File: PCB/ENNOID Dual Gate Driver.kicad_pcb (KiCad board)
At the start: 2 copper layers, 60 x 98 mm, 138 parts, among them J1 Conn_02x08_Odd_Even, J2 Current, J3 TEMP, J4 PHASE, J5 Collector, J6 Gate_H, J7 G_L, J8 E, M1 MountingHole_2.2mm_M2_Pad_Via, M2 MountingHole_2.2mm_M2_Pad_Via, M3 MountingHole_2.2mm_M2_Pad_Via, Q1 Q_NPN_BCE, Q2 Q_NPN_BCE, Q3 2N7002K-7, Q4 2N7002K-7, Q5 2N7002, Q6 2N7002, Q7 2N7002, Q8 2N7002, U1 MC7805, U2 MGJ2, U3 MGJ2, U4 1ED020I12-F2, U5 IXD-609, U6 1ED020I12-F2, U7 IXD-609, U8 AMC1301, U9 4069

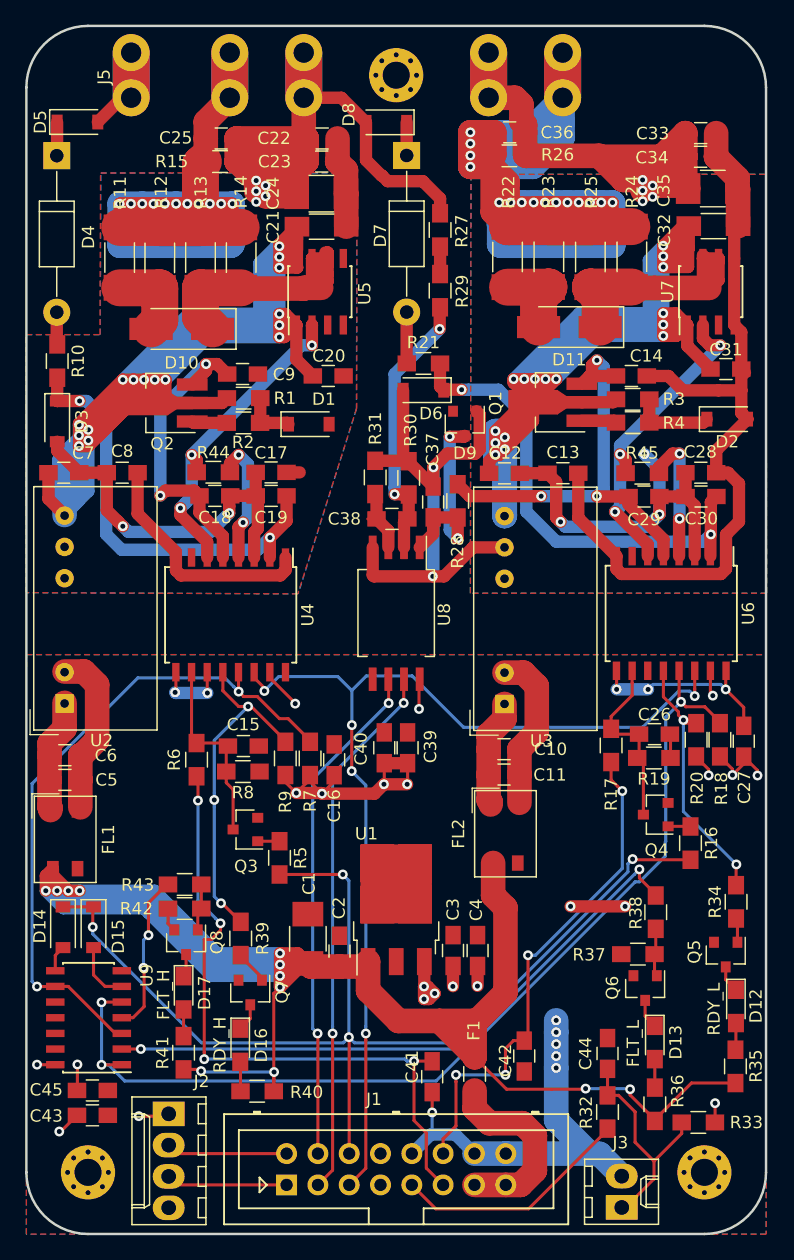
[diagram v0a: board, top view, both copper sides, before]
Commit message: PCB changes
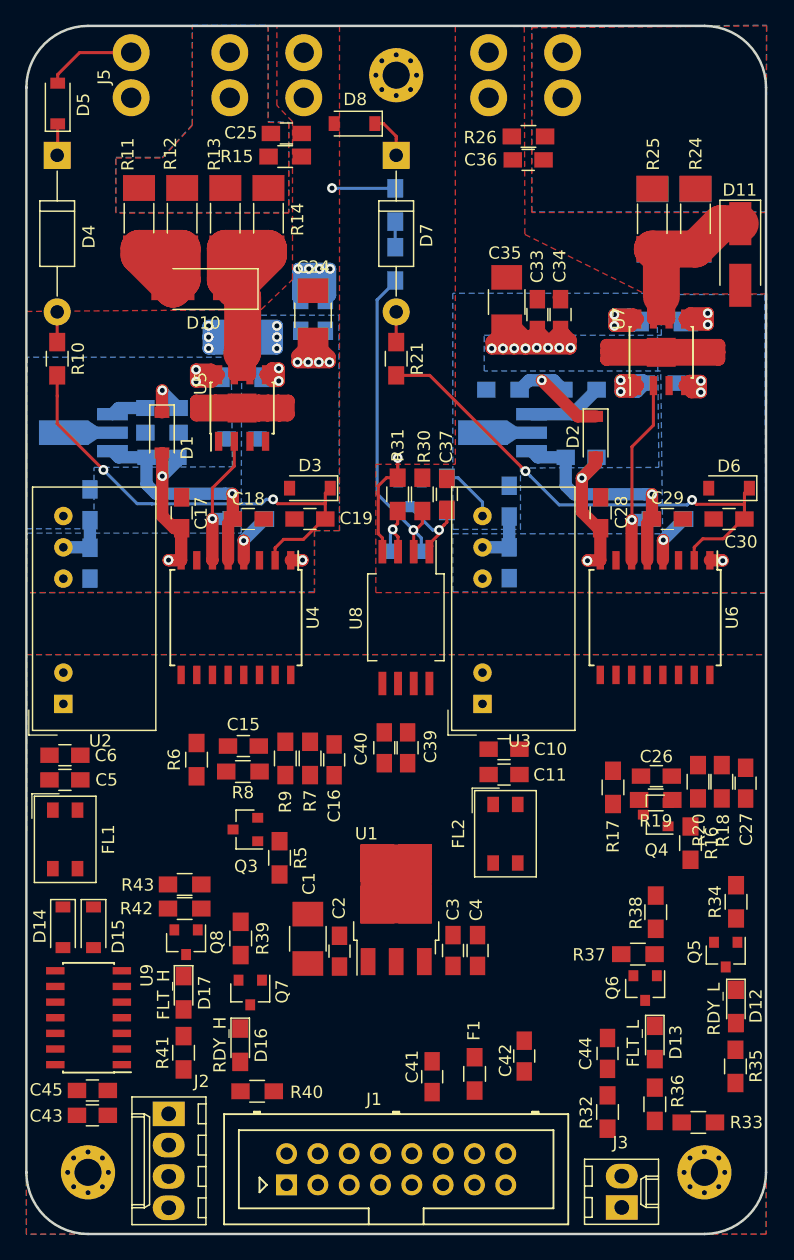
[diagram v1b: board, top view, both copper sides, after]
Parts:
- C12, C13, C14, C20, C21, C22, C23, C31, C32, C38, C7, C8, C9, D9, Q1, Q2, R1, R2, R22, R23, R27, R28, R29, R3, R4, R44, R45: moved to B.Cu
- R19, R8: value 1k -> 47k
- U5, U7: footprint Housings_SOIC:SOIC-8_3.9x4.9mm_Pitch1.27mm -> Housings_SOIC:SOIC-8-1EP_3.9x4.9mm_Pitch1.27mm
- moved D6 26.0 mm to (57.0, 37.5)
- moved D3 21.2 mm to (23.0, 37.5), turned to 180 degrees
- moved C33 19.8 mm to (41.5, 23.4), turned to 270 degrees
- moved C35 19.1 mm to (39.0, 22.4), turned to 270 degrees
- moved C34 17.1 mm to (43.3, 23.4), turned to 270 degrees
- moved D11 15.1 mm to (57.9, 18.5), turned to 270 degrees
- moved C22 14.4 mm to (24.3, 23.5), turned to 270 degrees
- moved C21 13.8 mm to (17.5, 28.5)
- moved C23 12.6 mm to (22.3, 23.5), turned to 270 degrees
- moved R23 12.3 mm to (54.3, 15.7)
- moved R22 12.1 mm to (50.8, 15.7)
- moved D1 11.9 mm to (11.0, 33.0), turned to 270 degrees
- moved U5 11.3 mm to (17.5, 31.0)
- moved D2 10.8 mm to (46.2, 33.3), turned to 270 degrees
- moved R3 10.6 mm to (38.7, 29.5)
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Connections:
- R28 pad 2: /GD_LOW/VCC_REG -> /GD_LOW/+VCC
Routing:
- net /GD_HIGH/+VCC: track 209.5 -> 5.02 mm, vias 16 -> 2
- net VCC_IN: track 182.9 -> 0.00 mm, vias 12 -> 0
- net /GD_LOW/+VCC: track 181.8 -> 25.1 mm, vias 16 -> 4
- net /GD_LOW/G: track 144.7 -> 0.00 mm, vias 15 -> 0
- net /GD_LOW/E: track 123.8 -> 15.8 mm, vias 10 -> 1
- net /GD_HIGH/G: track 93.5 -> 0.00 mm, vias 11 -> 0
- net FLT_ALL: track 91.8 -> 0.00 mm, vias 4 -> 0
- net RST: track 84.5 -> 0.00 mm, vias 5 -> 0
- net FLT_L: track 81.8 -> 0.00 mm, vias 3 -> 0
- net GND: track 62.1 -> 0.00 mm, vias 11 -> 0
- net +5V: track 61.7 -> 0.00 mm, vias 22 -> 0
- net FLT_H: track 55.9 -> 0.00 mm, vias 2 -> 0
- net PWM_H: track 54.2 -> 0.00 mm, vias 4 -> 0
- net (no net): track 0.00 -> 53.0 mm
- net Net-(R38-Pad1): track 50.7 -> 0.00 mm, vias 2 -> 0
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- added copper zone on B.Cu, net /GD_HIGH/+VCC
- added copper zone on B.Cu, net /GD_HIGH/-VEE
- added copper zone on B.Cu, net /GD_HIGH/G
- added copper zone on F.Cu, net /GD_HIGH/G
- added copper zone on B.Cu, net /GD_LOW/+VCC
- added copper zone on B.Cu, net /GD_LOW/-VEE
- added copper zone on F.Cu, net /GD_LOW/E
- added copper zone on B.Cu, net /GD_LOW/G
- added copper zone on F.Cu, net /GD_LOW/G
- added copper zone on F.Cu, net PHASE
- removed copper zone on F.Cu, net /GD_HIGH/-VEE
- removed copper zone on F.Cu, net /GD_LOW/-VEE
- removed copper zone on B.Cu, net /GD_LOW/E
- removed copper zone on B.Cu, net PHASE
